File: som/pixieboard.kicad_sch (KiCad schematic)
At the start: 16 parts, among them J1 Conn_02x20_Counter_Clockwise, J2 Conn_02x20_Counter_Clockwise, J3 Conn_02x20_Counter_Clockwise, J4 Conn_02x20_Counter_Clockwise, J5 Conn_02x20_Counter_Clockwise, J6 Conn_02x20_Counter_Clockwise, SW1 SW_DIP_x03, U1 XC7A200T-3FBG484E

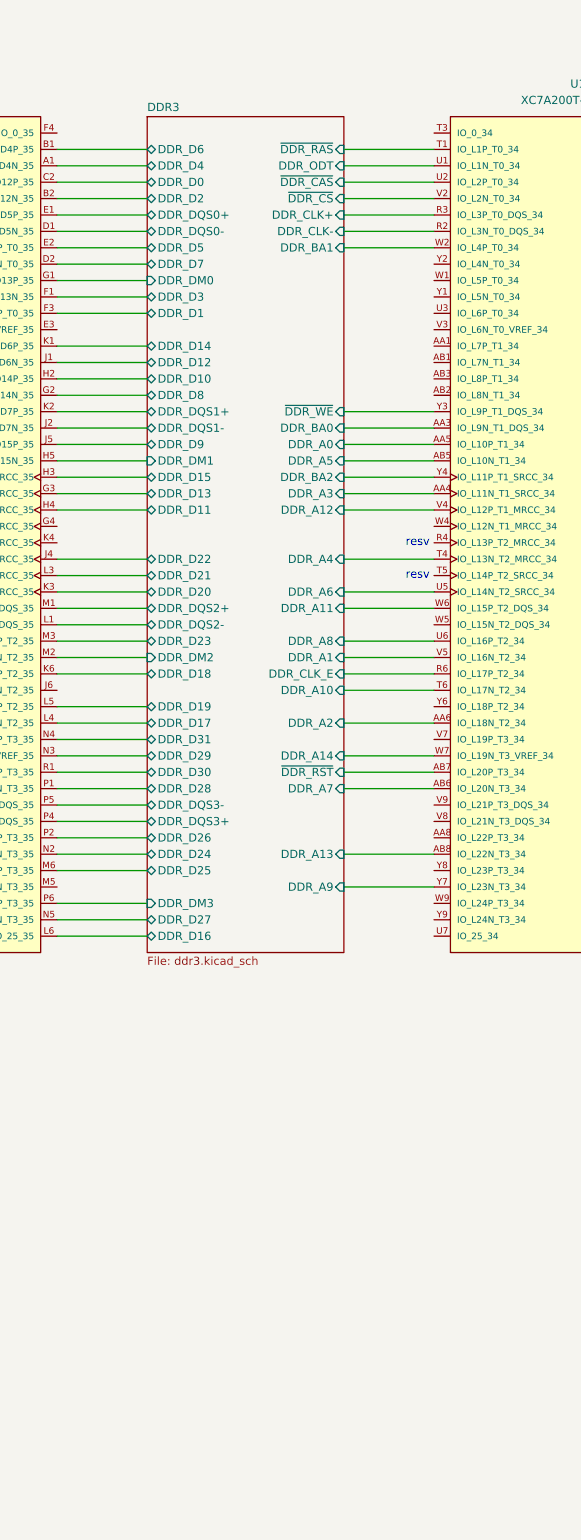
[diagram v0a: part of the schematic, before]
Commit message: ok
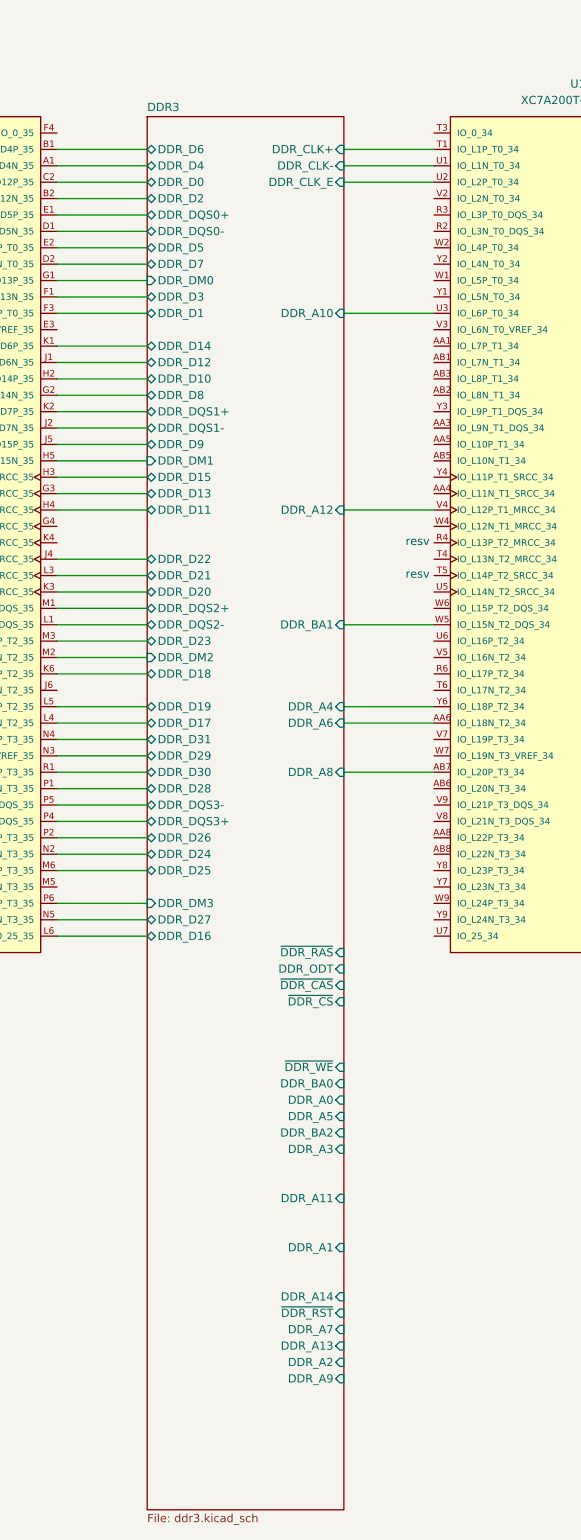
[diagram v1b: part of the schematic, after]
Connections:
- net DDR3/DDR_A0: no longer U1.AA5 (IO_L10P_T1_34)
- net DDR3/DDR_A1: no longer U1.V5 (IO_L16N_T2_34)
- net DDR3/DDR_A10: now also U1.U3 (IO_L6P_T0_34); no longer U1.T6 (IO_L17N_T2_34)
- net DDR3/DDR_A11: no longer U1.W6 (IO_L15P_T2_DQS_34)
- net DDR3/DDR_A13: no longer U1.AB8 (IO_L22N_T3_34)
- net DDR3/DDR_A14: no longer U1.W7 (IO_L19N_T3_VREF_34)
- net DDR3/DDR_A2: no longer U1.AA6 (IO_L18N_T2_34)
- net DDR3/DDR_A3: no longer U1.AA4 (IO_L11N_T1_SRCC_34)
- net DDR3/DDR_A4: now also U1.Y6 (IO_L18P_T2_34); no longer U1.T4 (IO_L13N_T2_MRCC_34)
- net DDR3/DDR_A5: no longer U1.AB5 (IO_L10N_T1_34)
- net DDR3/DDR_A6: now also U1.AA6 (IO_L18N_T2_34); no longer U1.U5 (IO_L14N_T2_SRCC_34)
- net DDR3/DDR_A7: no longer U1.AB6 (IO_L20N_T3_34)
- net DDR3/DDR_A8: now also U1.AB7 (IO_L20P_T3_34); no longer U1.U6 (IO_L16P_T2_34)
- net DDR3/DDR_A9: no longer U1.Y7 (IO_L23N_T3_34)
- net DDR3/DDR_BA0: no longer U1.AA3 (IO_L9N_T1_DQS_34)
- net DDR3/DDR_BA1: now also U1.W5 (IO_L15N_T2_DQS_34); no longer U1.W2 (IO_L4P_T0_34)
- net DDR3/DDR_BA2: no longer U1.Y4 (IO_L11P_T1_SRCC_34)
- net DDR3/DDR_CLK+: now also U1.T1 (IO_L1P_T0_34); no longer U1.R3 (IO_L3P_T0_DQS_34)
- net DDR3/DDR_CLK-: now also U1.U1 (IO_L1N_T0_34); no longer U1.R2 (IO_L3N_T0_DQS_34)
- net DDR3/DDR_CLK_E: now also U1.U2 (IO_L2P_T0_34); no longer U1.R6 (IO_L17P_T2_34)
- net DDR3/DDR_ODT: no longer U1.U1 (IO_L1N_T0_34)
- net DDR3/~{DDR_CAS}: no longer U1.U2 (IO_L2P_T0_34)
- net DDR3/~{DDR_CS}: no longer U1.V2 (IO_L2N_T0_34)
- net DDR3/~{DDR_RAS}: no longer U1.T1 (IO_L1P_T0_34)
- net DDR3/~{DDR_RST}: no longer U1.AB7 (IO_L20P_T3_34)
- net DDR3/~{DDR_WE}: no longer U1.Y3 (IO_L9P_T1_DQS_34)
